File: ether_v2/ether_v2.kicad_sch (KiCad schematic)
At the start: 82 parts, among them J1 PJ398SM, J10 PJ398SM, J11 PJ398SM, J12 PJ398SM, J13 PJ398SM, J14 PJ398SM, J15 PJ398SM, J16 PJ398SM, J17 SS65100-024F, J18 SS65100-024F, J2 PJ398SM, J20 Conn_01x03, J3 PJ398SM, J4 PJ398SM, J5 PJ398SM, J6 PJ398SM, J7 PJ398SM, J8 PJ398SM, J9 PJ398SM, J99 Power, U1 TL074, U2 TL074, U3 TL074, U4 TL074

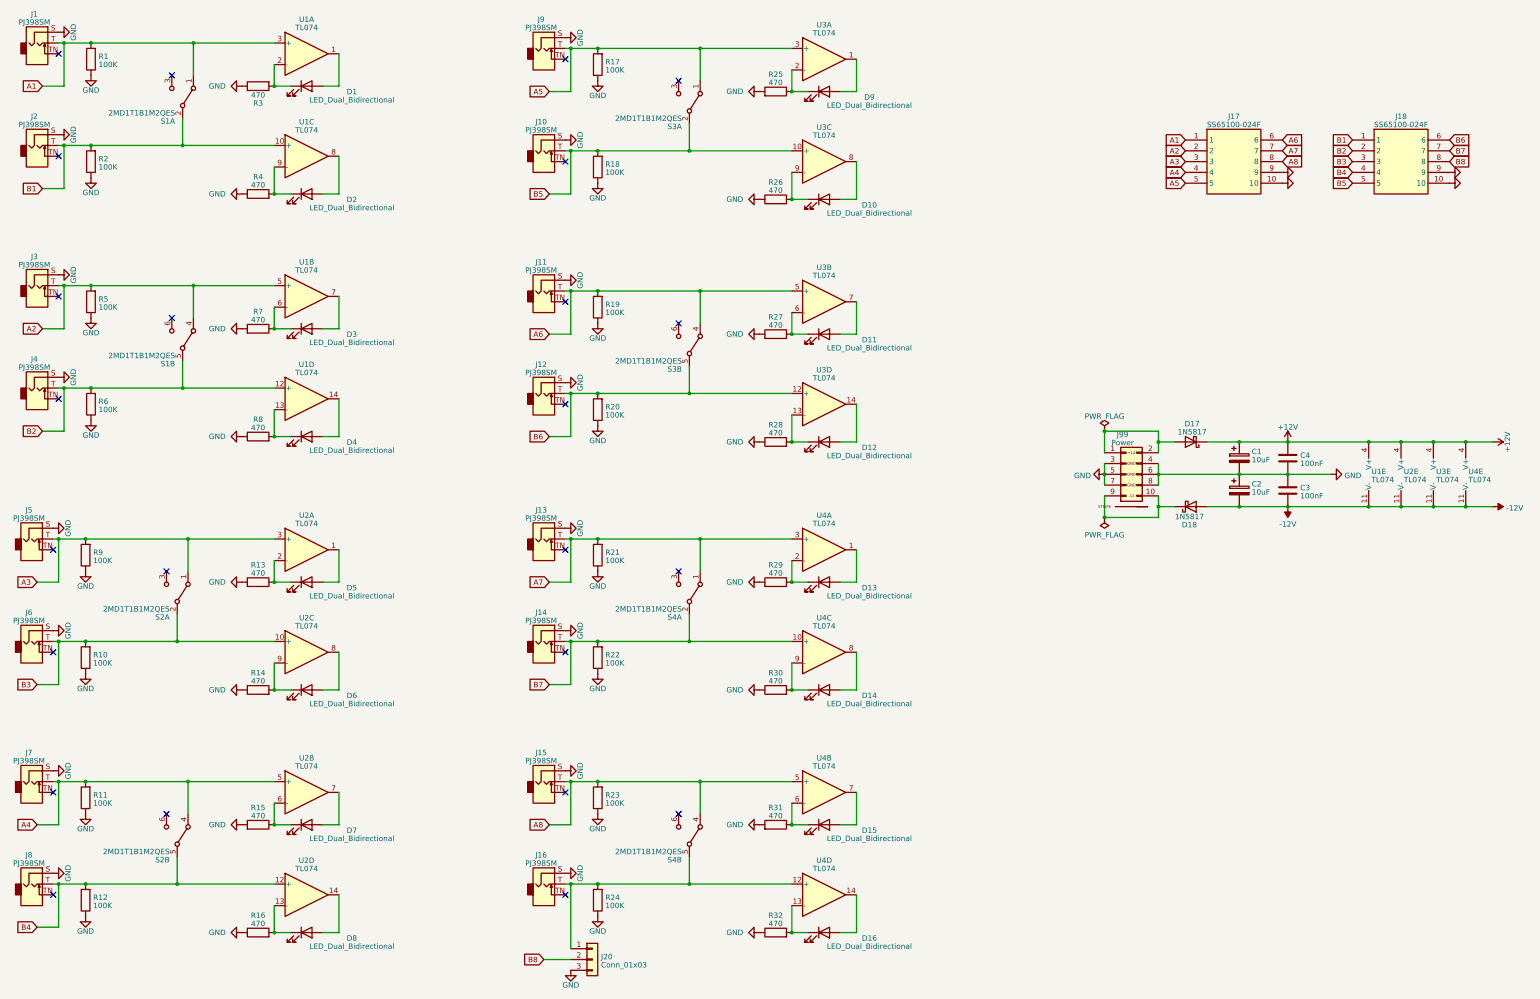
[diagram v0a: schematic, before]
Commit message: fix bad merge
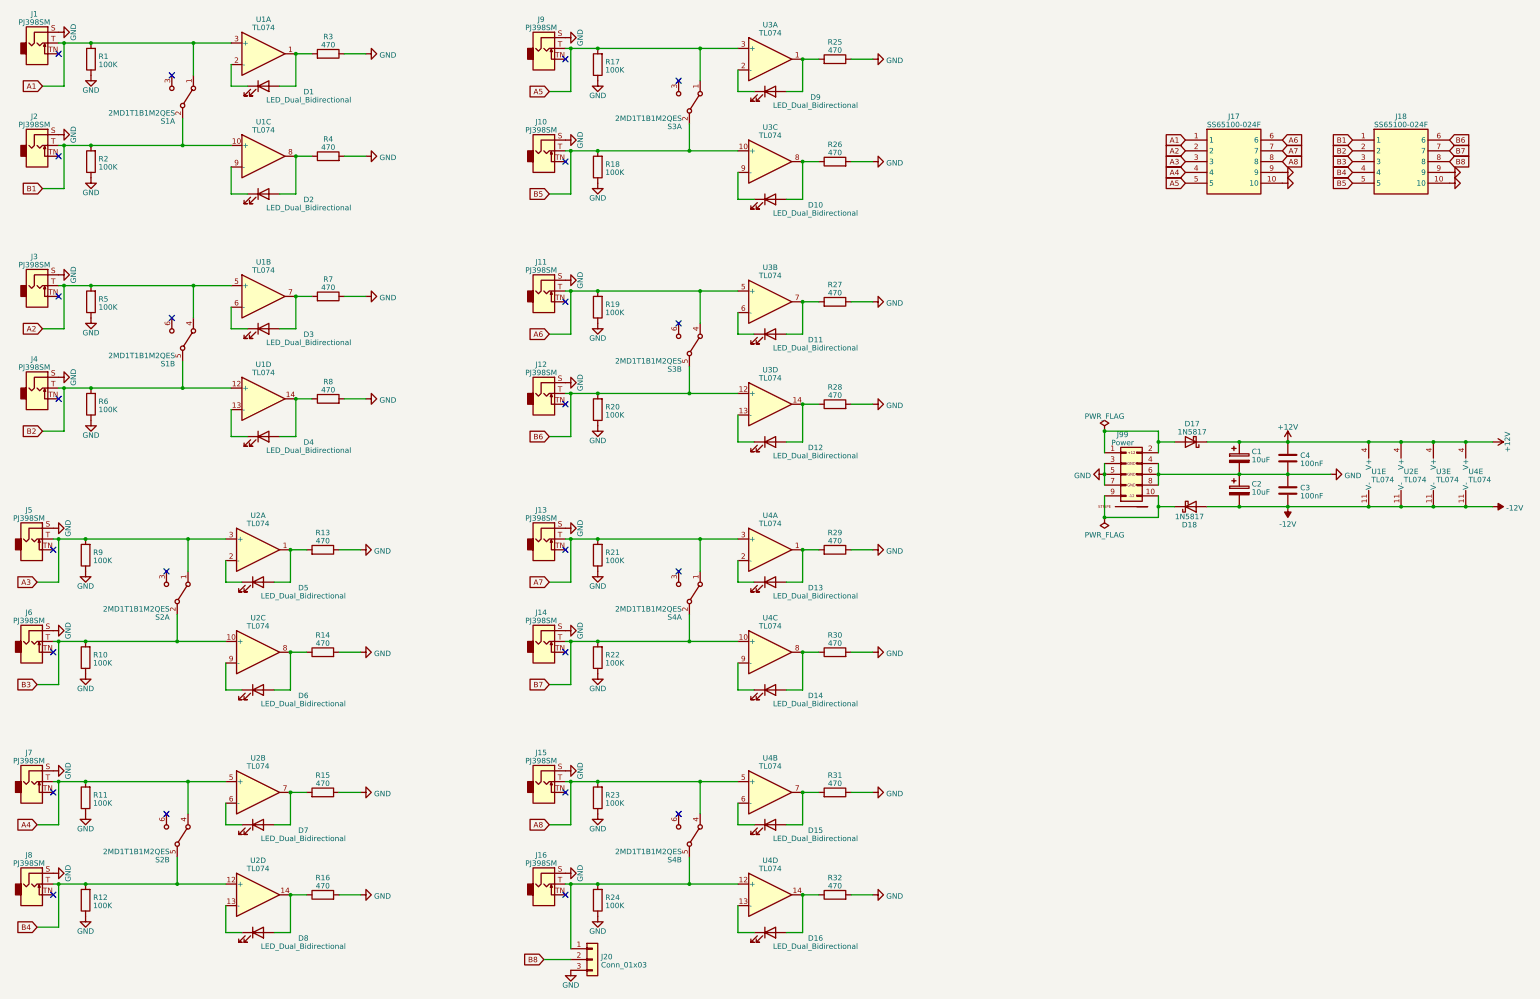
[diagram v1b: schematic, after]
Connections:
- net GND: now also R13.1, R14.2, R15.1, R16.2, R25.1, R26.2, R27.1, R28.2, R29.1, R30.2, R31.1, R32.2, R4.2, R7.1, R8.2; no longer R13.2, R14.1, R15.2, R16.1, R25.2, R26.1, R27.2, R28.1, R29.2, R30.1, R31.2, R32.1, R4.1, R7.2, R8.1
- net at D15.1 (K), U4.6 (-): no longer R31.1
- net at D15.2 (A), U4.7: now also R31.2
- net at D8.1 (K), U2.13 (-): no longer R16.2
- net at D8.2 (A), U2.14: now also R16.1
- net at D3.1 (K), U1.6 (-): no longer R7.1
- net at D7.1 (K), U2.6 (-): no longer R15.1
- net at D7.2 (A), U2.7: now also R15.2
- net at D14.2 (A), U4.8: now also R30.1
- net at D14.1 (K), U4.9 (-): no longer R30.2
- net at D1.2 (A), U1.1: now also R3.2
- net at D1.1 (K), U1.2 (-): no longer R3.2
- net at D11.1 (K), U3.6 (-): no longer R27.1
- net at D10.1 (K), U3.9 (-): no longer R26.2
- net at D10.2 (A), U3.8: now also R26.1
- net at D4.1 (K), U1.13 (-): no longer R8.2
- net at D4.2 (A), U1.14: now also R8.1
- net at D5.1 (K), U2.2 (-): no longer R13.1
- net at D5.2 (A), U2.1: now also R13.2
- net at D11.2 (A), U3.7: now also R27.2
- net at D2.1 (K), U1.9 (-): no longer R4.2
- net at D6.1 (K), U2.9 (-): no longer R14.2
- net at D2.2 (A), U1.8: now also R4.1
- net at D9.2 (A), U3.1: now also R25.2
- net at D9.1 (K), U3.2 (-): no longer R25.1
- net at D12.1 (K), U3.13 (-): no longer R28.2
- net at D12.2 (A), U3.14: now also R28.1
- net at D6.2 (A), U2.8: now also R14.1
- net at D3.2 (A), U1.7: now also R7.2
- net at D16.1 (K), U4.13 (-): no longer R32.2
- net at D16.2 (A), U4.14: now also R32.1
- net at D13.1 (K), U4.2 (-): no longer R29.1
- net at D13.2 (A), U4.1: now also R29.2
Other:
- moved on the sheet: D1, D10, D11, D12, D13, D14, D15, D16, D2, D3, D4, D5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
